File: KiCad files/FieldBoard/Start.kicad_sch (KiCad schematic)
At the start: 16 parts

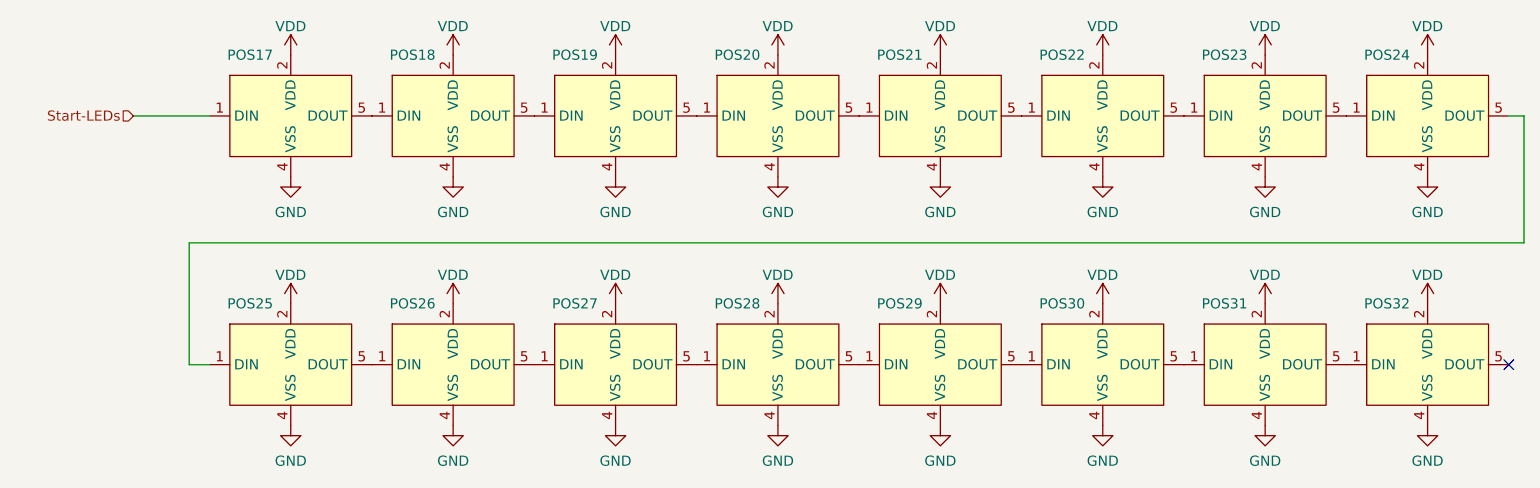
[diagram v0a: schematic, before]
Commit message: v2
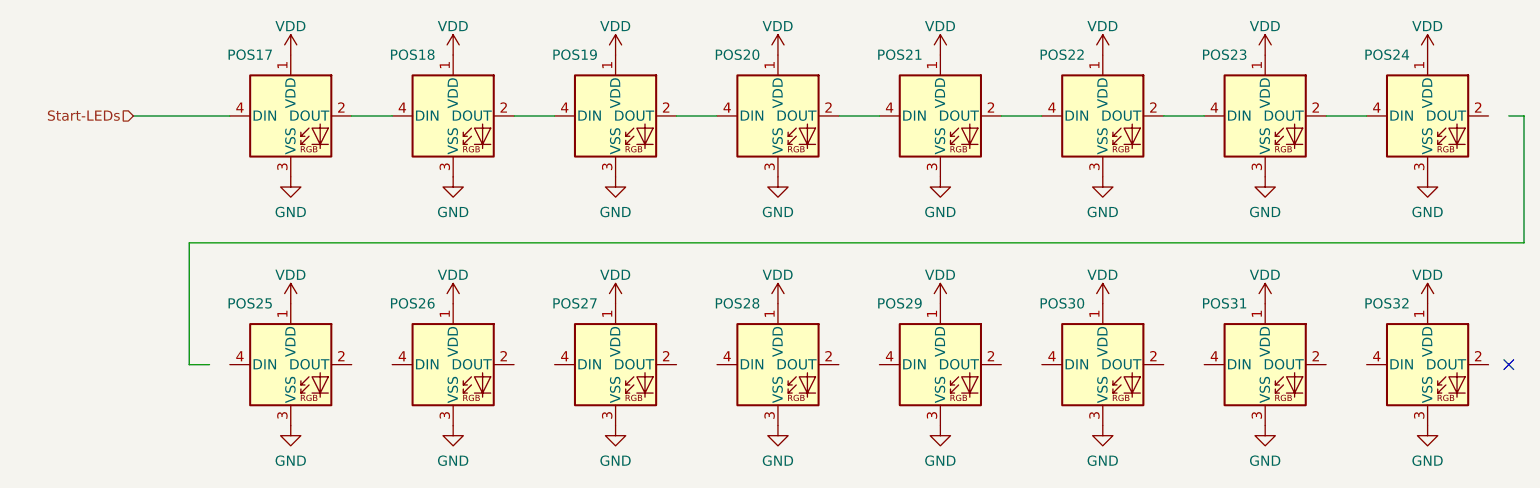
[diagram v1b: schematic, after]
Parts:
- POS17, POS18, POS19, POS20, POS21, POS22, POS23, POS24, POS25, POS26, POS27, POS28, POS29, POS30, POS31, POS32: footprint FieldBoard_footprint:WS2812-4020-dual-7mm_bezMaske -> LED_SMD:LED_WS2812B_PLCC4_5.0x5.0mm_P3.2mm; symbol FieldBoard_symbol:WS2812-4020_dual -> LED:WS2812B
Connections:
- net GND: now also POS17.3 (VSS), POS18.3 (VSS), POS19.3 (VSS), POS20.3 (VSS), POS21.3 (VSS), POS22.3 (VSS), POS23.3 (VSS), POS24.3 (VSS), POS25.3 (VSS), POS26.3 (VSS), POS27.3 (VSS), POS28.3 (VSS), POS29.3 (VSS), POS30.3 (VSS), POS31.3 (VSS), POS32.3 (VSS); no longer POS17.4 (VSS), POS18.4 (VSS), POS19.4 (VSS), POS20.4 (VSS), POS21.4 (VSS), POS22.4 (VSS), POS23.4 (VSS), POS24.4 (VSS), POS25.4 (VSS), POS26.4 (VSS), POS27.4 (VSS), POS28.4 (VSS), POS29.4 (VSS), POS30.4 (VSS), POS31.4 (VSS), POS32.4 (VSS)
- net Start-LEDs: now also POS17.4 (DIN); no longer POS17.1 (DIN)
- net VDD: now also POS17.1 (VDD), POS18.1 (VDD), POS19.1 (VDD), POS20.1 (VDD), POS21.1 (VDD), POS22.1 (VDD), POS23.1 (VDD), POS24.1 (VDD), POS25.1 (VDD), POS26.1 (VDD), POS27.1 (VDD), POS28.1 (VDD), POS29.1 (VDD), POS30.1 (VDD), POS31.1 (VDD), POS32.1 (VDD); no longer POS17.2 (VDD), POS18.2 (VDD), POS19.2 (VDD), POS20.2 (VDD), POS21.2 (VDD), POS22.2 (VDD), POS23.2 (VDD), POS24.2 (VDD), POS25.2 (VDD), POS26.2 (VDD), POS27.2 (VDD), POS28.2 (VDD), POS29.2 (VDD), POS30.2 (VDD), POS31.2 (VDD), POS32.2 (VDD)
- new net: POS20.2 (DOUT), POS21.4 (DIN)
- new net: POS19.2 (DOUT), POS20.4 (DIN)
- new net: POS21.2 (DOUT), POS22.4 (DIN)
- new net: POS23.2 (DOUT), POS24.4 (DIN)
- new net: POS18.2 (DOUT), POS19.4 (DIN)
- new net: POS17.2 (DOUT), POS18.4 (DIN)
- new net: POS22.2 (DOUT), POS23.4 (DIN)
